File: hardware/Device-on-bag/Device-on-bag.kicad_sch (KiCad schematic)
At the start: 4 parts, among them J1 Conn_01x08, J2 Conn_01x08, U1 SparkFun_SEN-14480_H3LIS331DL, U2 ESP32-DEVKIT-V1

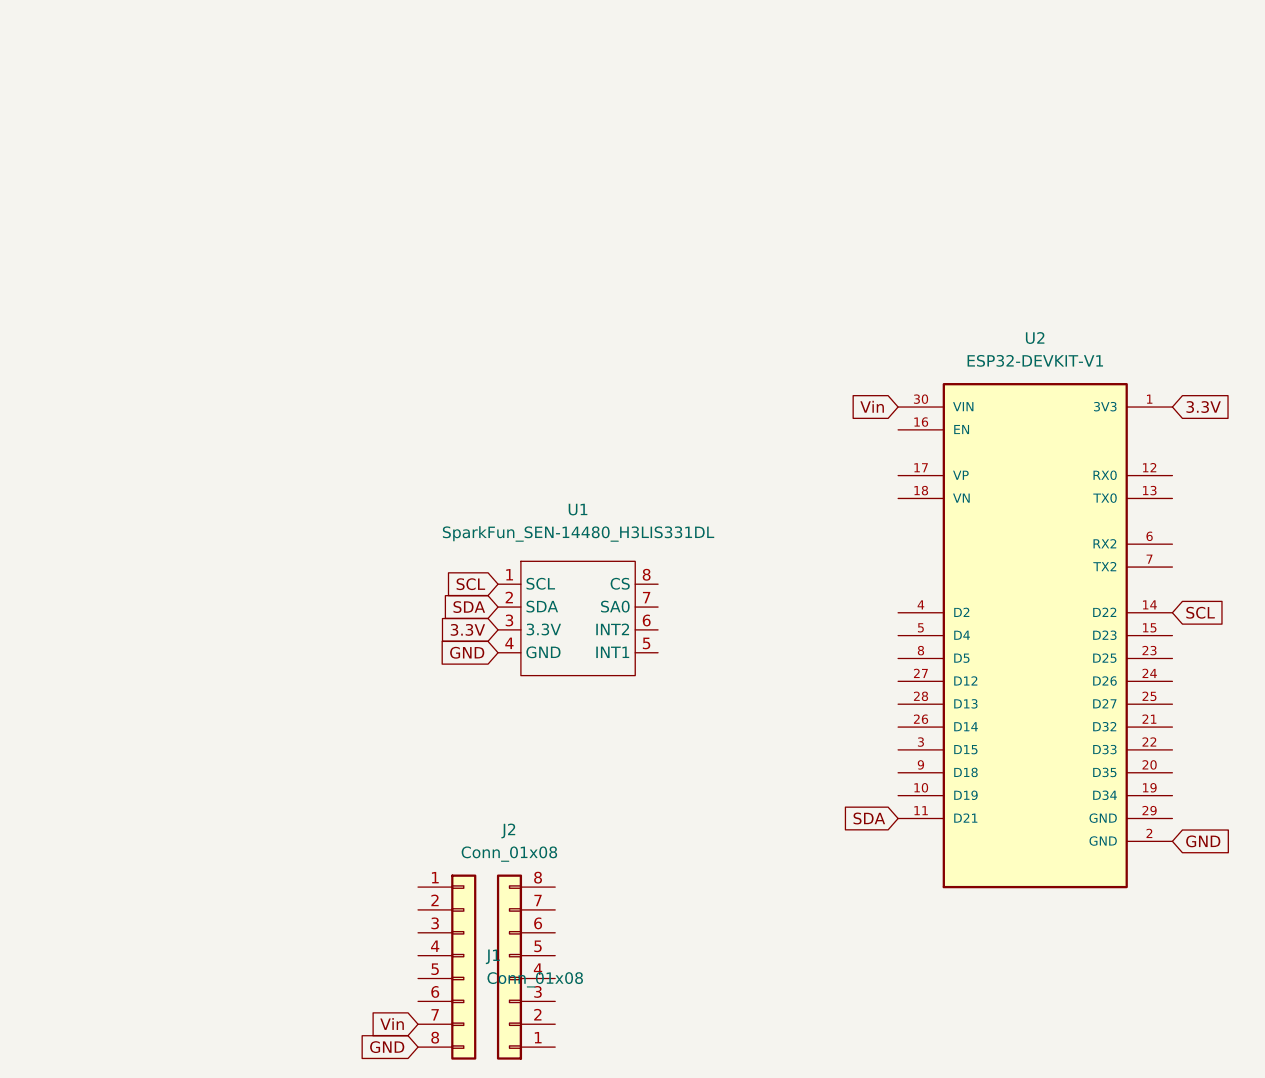
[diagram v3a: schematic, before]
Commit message: update
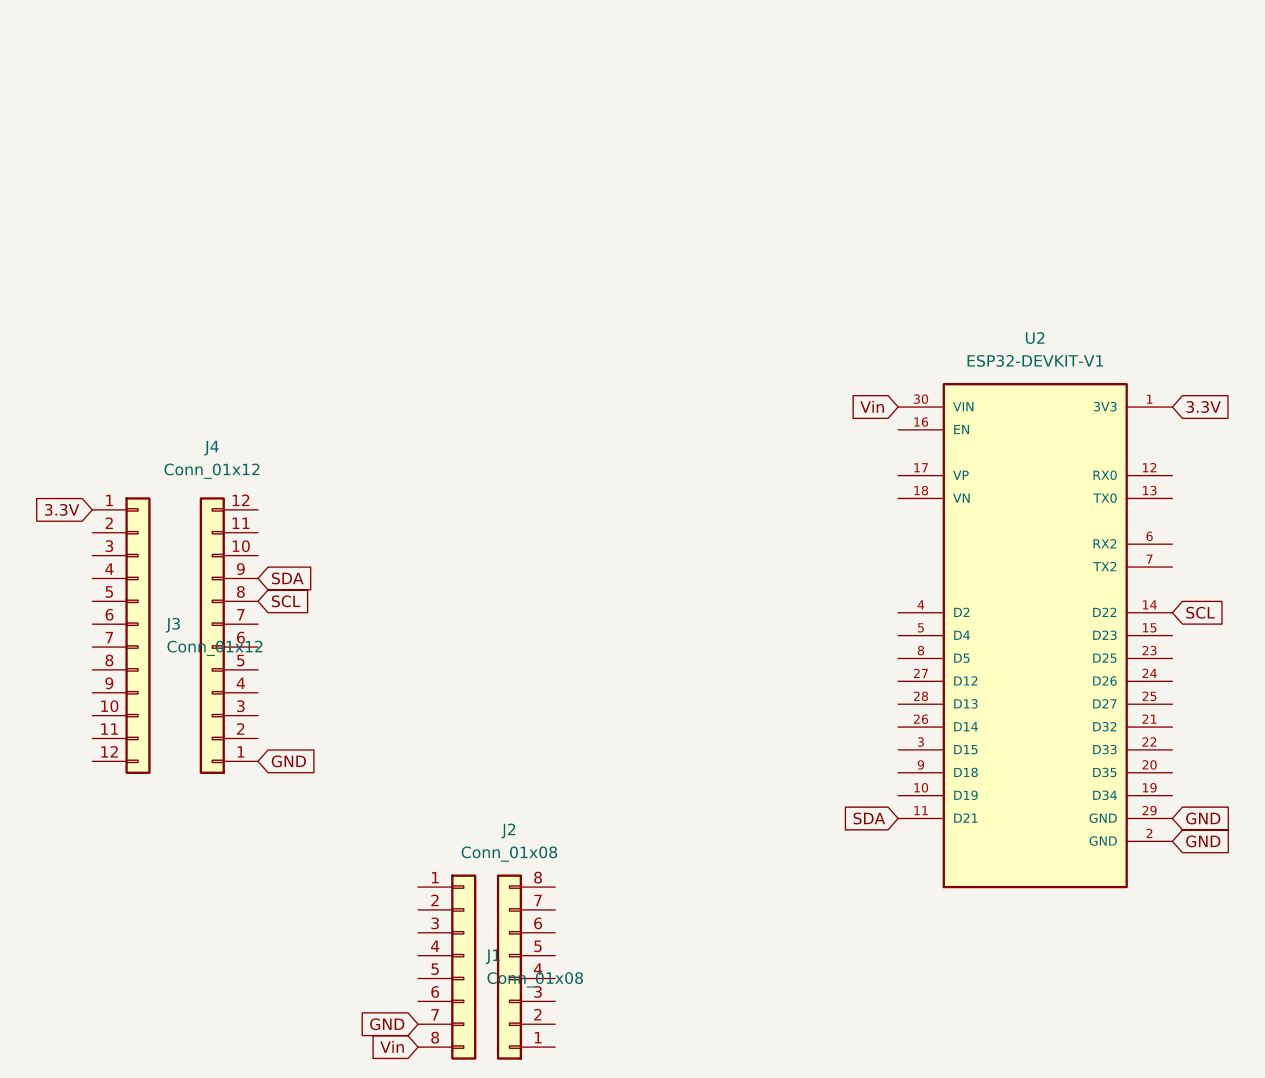
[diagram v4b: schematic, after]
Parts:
- removed U1: SparkFun_SEN-14480_H3LIS331DL, SparkFun_Tri_Axis_Accel_Breakout-H3LIS331DL:SparkFun_Tri_Axis_Accel_Breakout-H3LIS331DL, symbol H3LIS331DL:SparkFun_SEN-14480_H3LIS331DL
- added J3, J4: Conn_01x12, Connector_PinSocket_2.54mm:PinSocket_1x12_P2.54mm_Vertical, symbol Connector_Generic:Conn_01x12
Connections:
- net 3.3V: now also J3.1 (Pin_1)
- net GND: now also J1.7 (Pin_7), U2.29 (GND), J4.1 (Pin_1); no longer J1.8 (Pin_8)
- net SCL: now also J4.8 (Pin_8)
- net SDA: now also J4.9 (Pin_9)
- net Vin: now also J1.8 (Pin_8); no longer J1.7 (Pin_7)
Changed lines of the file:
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@@
 (kicad_sch (version 20211123) (generator eeschema)
   (paper "A4")
-  (global_label "3.3V" (shape input) (at 118.11 98.425 180) (fields_autoplaced)
-    (effects (font (size 1.27 1.27)) (justify right))
-    (property "Intersheet References" "${INTERSHEET_REFS}" (id 0) (at 111.5845 98.5044 0)
-      (effects (font (size 1.27 1.27)) (justify right) hide)
-    )
-  )
-  (global_label "Vin" (shape input) (at 109.22 142.24 180) (fields_autoplaced)
-    (effects (font (size 1.27 1.27)) (justify right))
-    (property "Intersheet References" "${INTERSHEET_REFS}" (id 0) (at 103.9645 142.1606 0)
+  (global_label "SDA" (shape input) (at 91.44 92.71 0) (fields_autoplaced)
+    (effects (font (size 1.27 1.27)) (justify left))
+    (property "Intersheet References" "${INTERSHEET_REFS}" (id 0) (at 97.4212 92.6306 0)
+      (effects (font (size 1.27 1.27)) (justify left) hide)
+    )
+  )
+  (global_label "GND" (shape input) (at 193.04 119.38 0) (fields_autoplaced)
+    (effects (font (size 1.27 1.27)) (justify left))
+    (property "Intersheet References" "${INTERSHEET_REFS}" (id 0) (at 199.3236 119.4594 0)
+      (effects (font (size 1.27 1.27)) (justify left) hide)
+    )
+  )
+  (global_label "Vin" (shape input) (at 109.22 144.78 180) (fields_autoplaced)
+    (effects (font (size 1.27 1.27)) (justify right))
+    (property "Intersheet References" "${INTERSHEET_REFS}" (id 0) (at 103.9645 144.7006 0)
       (effects (font (size 1.27 1.27)) (justify right) hide)
     )
@@
     )
   )
-  (global_label "GND" (shape input) (at 118.11 100.965 180) (fields_autoplaced)
-    (effects (font (size 1.27 1.27)) (justify right))
-    (property "Intersheet References" "${INTERSHEET_REFS}" (id 0) (at 111.8264 100.8856 0)
-      (effects (font (size 1.27 1.27)) (justify right) hide)
+  (global_label "GND" (shape input) (at 91.44 113.03 0) (fields_autoplaced)
+    (effects (font (size 1.27 1.27)) (justify left))
+    (property "Intersheet References" "${INTERSHEET_REFS}" (id 0) (at 97.7236 113.1094 0)
+      (effects (font (size 1.27 1.27)) (justify left) hide)
     )
   )
@@
     )
   )
-  (global_label "GND" (shape input) (at 109.22 144.78 180) (fields_autoplaced)
-    (effects (font (size 1.27 1.27)) (justify right))
-    (property "Intersheet References" "${INTERSHEET_REFS}" (id 0) (at 102.9364 144.7006 0)
+  (global_label "GND" (shape input) (at 109.22 142.24 180) (fields_autoplaced)
+    (effects (font (size 1.27 1.27)) (justify right))
+    (property "Intersheet References" "${INTERSHEET_REFS}" (id 0) (at 102.9364 142.1606 0)
       (effects (font (size 1.27 1.27)) (justify right) hide)
     )
@@
     )
   )
+  (global_label "3.3V" (shape input) (at 73.025 85.09 180) (fields_autoplaced)
+    (effects (font (size 1.27 1.27)) (justify right))
+    (property "Intersheet References" "${INTERSHEET_REFS}" (id 0) (at 66.4995 85.1694 0)
+      (effects (font (size 1.27 1.27)) (justify right) hide)
+    )
+  )
   (global_label "SDA" (shape input) (at 162.56 119.38 180) (fields_autoplaced)
     (effects (font (size 1.27 1.27)) (justify right))
@@
     )
   )
-  (global_label "SCL" (shape input) (at 118.11 93.345 180) (fields_autoplaced)
-    (effects (font (size 1.27 1.27)) (justify right))
-    (property "Intersheet References" "${INTERSHEET_REFS}" (id 0) (at 112.1893 93.4244 0)
-      (effects (font (size 1.27 1.27)) (justify right) hide)
+  (global_label "SCL" (shape input) (at 91.44 95.25 0) (fields_autoplaced)
+    (effects (font (size 1.27 1.27)) (justify left))
+    (property "Intersheet References" "${INTERSHEET_REFS}" (id 0) (at 97.3607 95.1706 0)
+      (effects (font (size 1.27 1.27)) (justify left) hide)
     )
   )
@@
     (property "Intersheet References" "${INTERSHEET_REFS}" (id 0) (at 198.9607 96.4406 0)
       (effects (font (size 1.27 1.27)) (justify left) hide)
-    )
-  )
-  (global_label "SDA" (shape input) (at 118.11 95.885 180) (fields_autoplaced)
-    (effects (font (size 1.27 1.27)) (justify right))
-    (property "Intersheet References" "${INTERSHEET_REFS}" (id 0) (at 112.1288 95.9644 0)
-      (effects (font (size 1.27 1.27)) (justify right) hide)
     )
   )
@@
     (pin "8")
   )
+  (symbol (lib_id "Connector_Generic:Conn_01x12") (at 78.105 97.79 0) (unit 1)
+    (in_bom yes) (on_board yes) (fields_autoplaced)
+    (property "Reference" "J3" (id 0) (at 81.28 97.7899 0)
+      (effects (font (size 1.27 1.27)) (justify left))
+    )
+    (property "Value" "Conn_01x12" (id 1) (at 81.28 100.3299 0)
+      (effects (font (size 1.27 1.27)) (justify left))
+    )
+    (property "Footprint" "Connector_PinSocket_2.54mm:PinSocket_1x12_P2.54mm_Vertical" (id 2) (at 78.105 97.79 0)
+      (effects (font (size 1.27 1.27)) hide)
+    )
+    (property "Datasheet" "~" (id 3) (at 78.105 97.79 0)
+      (effects (font (size 1.27 1.27)) hide)
+    )
+    (pin "1")
+    (pin "10")
+    (pin "11")
+    (pin "12")
+    (pin "2")
+    (pin "3")
+    (pin "4")
+    (pin "5")
+    (pin "6")
+    (pin "7")
+    (pin "8")
+    (pin "9")
+  )
   (symbol (lib_id "Connector_Generic:Conn_01x08") (at 114.3 134.62 0) (unit 1)
     (in_bom yes) (on_board yes) (fields_autoplaced)
@@
     (pin "8")
   )
-  (symbol (lib_id "H3LIS331DL:SparkFun_SEN-14480_H3LIS331DL") (at 127 97.155 0) (unit 1)
-    (in_bom yes) (on_board yes) (fields_autoplaced)
-    (property "Reference" "U1" (id 0) (at 127 85.09 0))
-    (property "Value" "SparkFun_SEN-14480_H3LIS331DL" (id 1) (at 127 87.63 0))
-    (property "Footprint" "SparkFun_Tri_Axis_Accel_Breakout-H3LIS331DL:SparkFun_Tri_Axis_Accel_Breakout-H3LIS331DL" (id 2) (at 127 97.155 0)
-      (effects (font (size 1.27 1.27)) hide)
-    )
-    (property "Datasheet" "" (id 3) (at 127 97.155 0)
-      (effects (font (size 1.27 1.27)) hide)
-    )
-    (pin "1")
-    (pin "2")
-    (pin "3")
-    (pin "4")
-    (pin "5")
-    (pin "6")
-    (pin "7")
-    (pin "8")
+  (symbol (lib_id "Connector_Generic:Conn_01x12") (at 86.36 100.33 180) (unit 1)
+    (in_bom yes) (on_board yes) (fields_autoplaced)
+    (property "Reference" "J4" (id 0) (at 86.36 78.105 0))
+    (property "Value" "Conn_01x12" (id 1) (at 86.36 80.645 0))
+    (property "Footprint" "Connector_PinSocket_2.54mm:PinSocket_1x12_P2.54mm_Vertical" (id 2) (at 86.36 100.33 0)
+      (effects (font (size 1.27 1.27)) hide)
+    )
+    (property "Datasheet" "~" (id 3) (at 86.36 100.33 0)
+      (effects (font (size 1.27 1.27)) hide)
+    )
+    (pin "1")
+    (pin "10")
+    (pin "11")
+    (pin "12")
+    (pin "2")
+    (pin "3")
+    (pin "4")
+    (pin "5")
+    (pin "6")
+    (pin "7")
+    (pin "8")
+    (pin "9")
   )
   (symbol (lib_id "ESP32-DEVKIT-V1:ESP32-DEVKIT-V1") (at 177.8 99.06 0) (unit 1)
@@
       (reference "J2") (unit 1) (value "Conn_01x08") (footprint "Connector_PinSocket_2.54mm:PinSocket_1x08_P2.54mm_Vertical")
     )
-    (path "/bdadbb5c-7221-4007-9a12-2ce8f2e20049"
-      (reference "U1") (unit 1) (value "SparkFun_SEN-14480_H3LIS331DL") (footprint "SparkFun_Tri_Axis_Accel_Breakout-H3LIS331DL:SparkFun_Tri_Axis_Accel_Breakout-H3LIS331DL")
+    (path "/752f9595-3eb9-4010-a3c3-154e60e73472"
+      (reference "J3") (unit 1) (value "Conn_01x12") (footprint "Connector_PinSocket_2.54mm:PinSocket_1x12_P2.54mm_Vertical")
+    )
+    (path "/ec14a061-dfd4-4b23-b005-a6397276b0b5"
+      (reference "J4") (unit 1) (value "Conn_01x12") (footprint "Connector_PinSocket_2.54mm:PinSocket_1x12_P2.54mm_Vertical")
     )
     (path "/f3434164-7b41-4e11-b256-2613206fdd17"
